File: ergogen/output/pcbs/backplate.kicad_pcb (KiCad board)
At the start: 2 copper layers, 139.5 x 113.2 mm, 5 parts

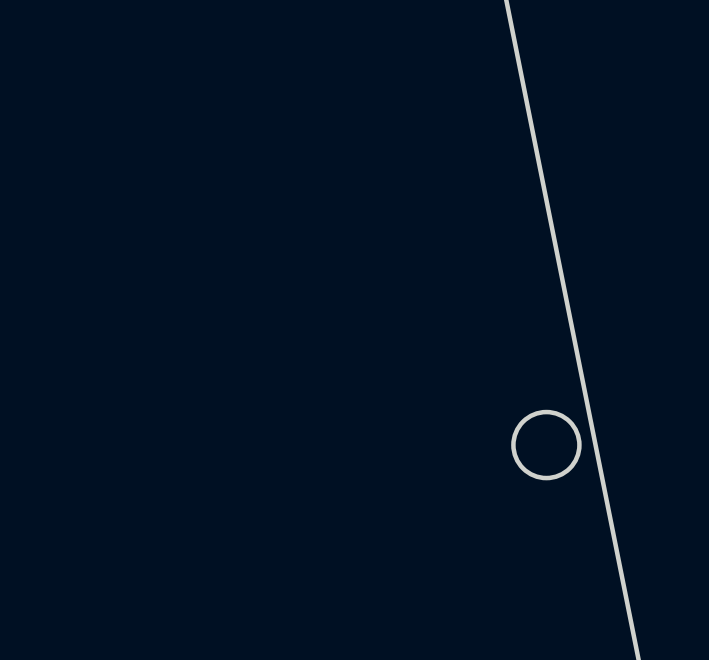
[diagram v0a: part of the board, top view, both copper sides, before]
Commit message: Checkpoint
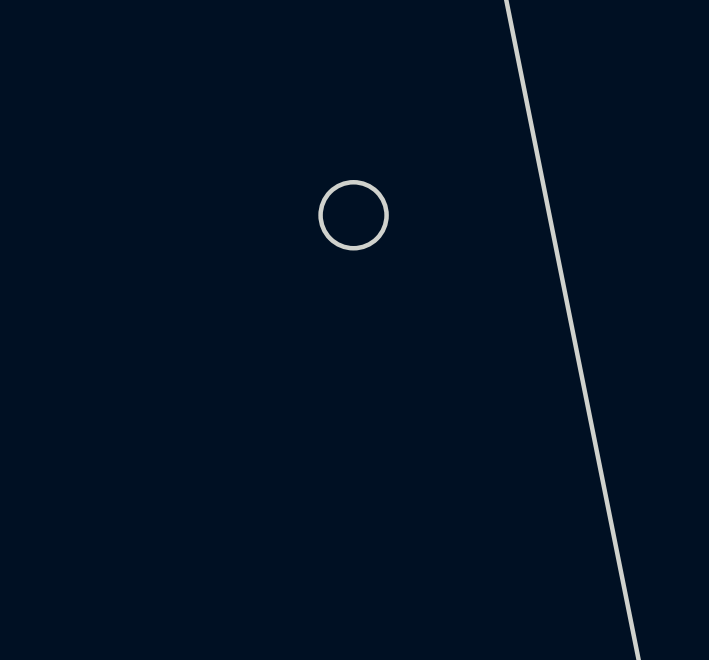
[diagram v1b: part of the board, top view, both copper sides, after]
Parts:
- moved MH5 10.00 mm to (220.8, 121.4)
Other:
- outline, holes or cut-outs redrawn
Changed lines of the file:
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@@
   )
   (module "ceoloide:mounting_hole_npth" (layer F.Cu)
-      (at 227.2307082 129.0614476 -50)
+      (at 220.8028321 121.40100319999999 -50)
       (fp_text reference "MH5" (at 0 2.55 -50) (layer F.SilkS) hide (effects (font (size 1 1) (thickness 0.15))))
       (pad "" np_thru_hole circle (at 0 0 -50) (size 2.2 2.2) (drill 2.2) (layers *.Cu *.Mask))
@@
 (gr_circle (center 185.468 61.361000000000004) (end 186.56799999999998 61.361000000000004) (layer Edge.Cuts) (width 0.15))
 (gr_circle (center 172.7442902 101.1746489) (end 173.8442902 101.1746489) (layer Edge.Cuts) (width 0.15))
-(gr_circle (center 227.2307082 129.0614476) (end 228.3307082 129.0614476) (layer Edge.Cuts) (width 0.15))
+(gr_circle (center 220.8028321 121.40100319999999) (end 221.90283209999998 121.40100319999999) (layer Edge.Cuts) (width 0.15))
 )

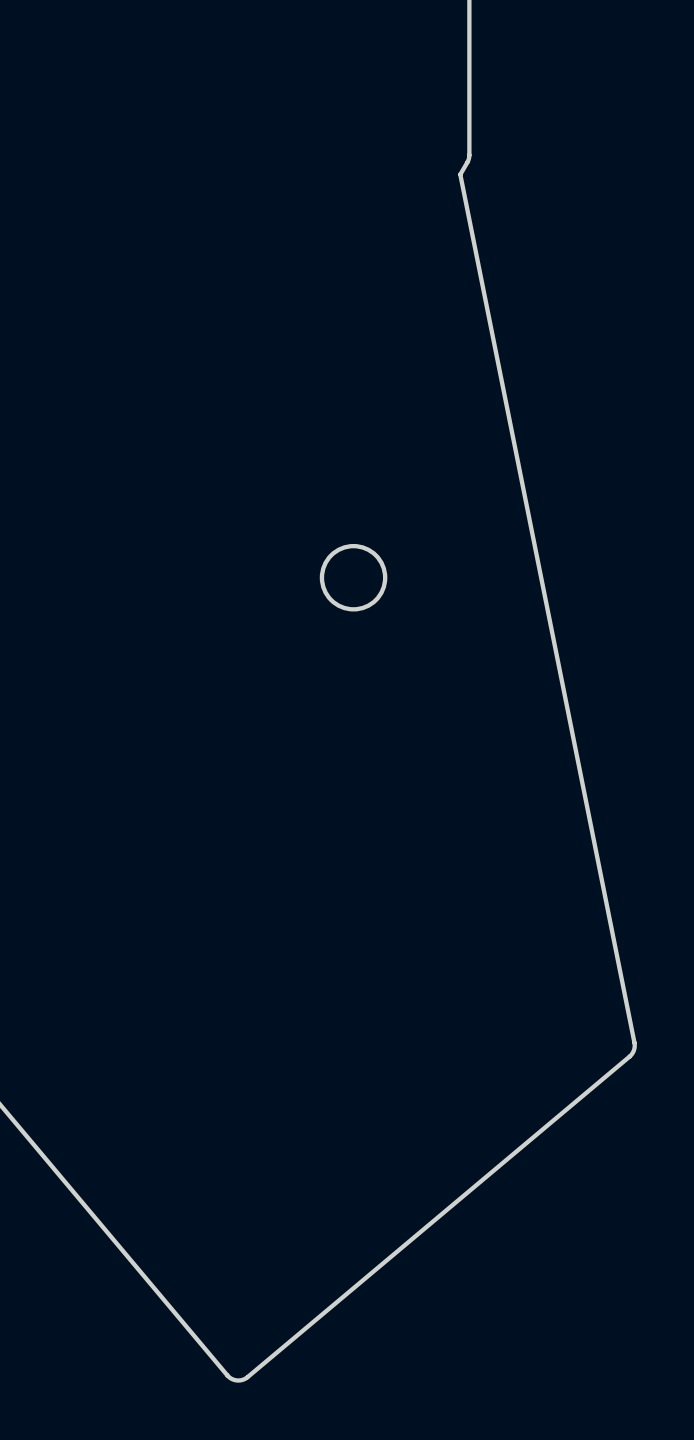
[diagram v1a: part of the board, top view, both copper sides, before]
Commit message: Checkpoint
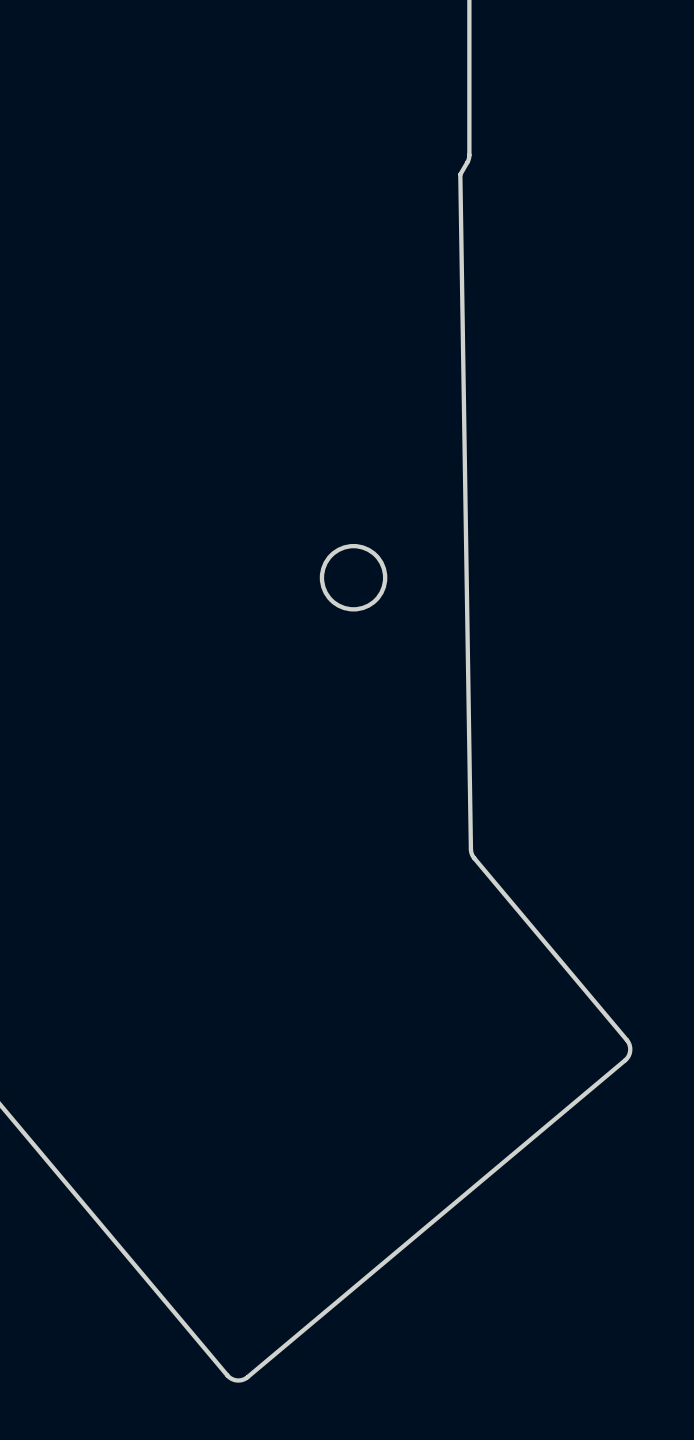
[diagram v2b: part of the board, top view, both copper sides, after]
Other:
- board size 139.5 x 113.2 mm -> 139.4 x 113.2 mm
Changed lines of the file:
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@@
 (gr_line (start 185.58186840000002 44.10813154431579) (end 203.5823534679014 44.1128685140705) (angle 90) (layer Edge.Cuts) (width 0.15))
 (gr_line (start 204.08222186790144 44.61264651408419) (end 204.08277807371226 45.86522200005129) (angle 90) (layer Edge.Cuts) (width 0.15))
-(gr_line (start 224.518 107.371596) (end 230.57788045934674 137.5834997388322) (angle 90) (layer Edge.Cuts) (width 0.15))
-(gr_line (start 230.40903856128045 138.06485304847308) (end 217.11551321531311 149.21944520216027) (angle 90) (layer Edge.Cuts) (width 0.15))
+(gr_line (start 224.518 107.371596) (end 224.88688692725793 130.84827901796234) (angle 90) (layer Edge.Cuts) (width 0.15))
+(gr_line (start 225.00380302725722 131.16181731796115) (end 230.3148039002676 137.491221684766) (angle 90) (layer Edge.Cuts) (width 0.15))
+(gr_line (start 230.25317550026756 138.19563768476607) (end 217.1155132153131 149.21944520216027) (angle 90) (layer Edge.Cuts) (width 0.15))
 (gr_line (start 216.41109721531305 149.1578168021602) (end 205.28039649130588 135.89276421578668) (angle 90) (layer Edge.Cuts) (width 0.15))
 (gr_line (start 205.18757259130587 135.8069910157867) (end 189.74612938848182 124.80148031587586) (angle 90) (layer Edge.Cuts) (width 0.15))
@@
 (gr_arc (start 224.333 46.865) (end 224.833 46.865) (angle -90) (layer Edge.Cuts) (width 0.15))
 (gr_arc (start 224.333 106.69202540612952) (end 224.7660127 106.94202540612952) (angle -30.000000108401252) (layer Edge.Cuts) (width 0.15))
-(gr_arc (start 230.0876447612805 137.68183084847306) (end 230.4090385612805 138.06485304847305) (angle -61.34183996214843) (layer Edge.Cuts) (width 0.15))
-(gr_arc (start 216.7941194153131 148.83642300216025) (end 216.4110972153131 149.15781680216026) (angle -90.00000000000713) (layer Edge.Cuts) (width 0.15))
+(gr_arc (start 225.3868252272579 130.84042351796052) (end 224.8868869272579 130.84827901796052) (angle -39.099790156987126) (layer Edge.Cuts) (width 0.15))
+(gr_arc (start 229.93178170026758 137.812615484766) (end 230.2531755002676 138.195637684766) (angle -90.00000000000456) (layer Edge.Cuts) (width 0.15))
+(gr_arc (start 216.79411941531308 148.83642300216025) (end 216.41109721531308 149.15781680216026) (angle -90.00000000000503) (layer Edge.Cuts) (width 0.15))
 (gr_arc (start 204.8973742913059 136.21415801578672) (end 205.2803964913059 135.8927642157867) (angle -14.521558200128908) (layer Edge.Cuts) (width 0.15))
 (gr_arc (start 189.45593108848183 125.20864731587585) (end 189.74612938848182 124.80148031587585) (angle -15.00000020686845) (layer Edge.Cuts) (width 0.15))

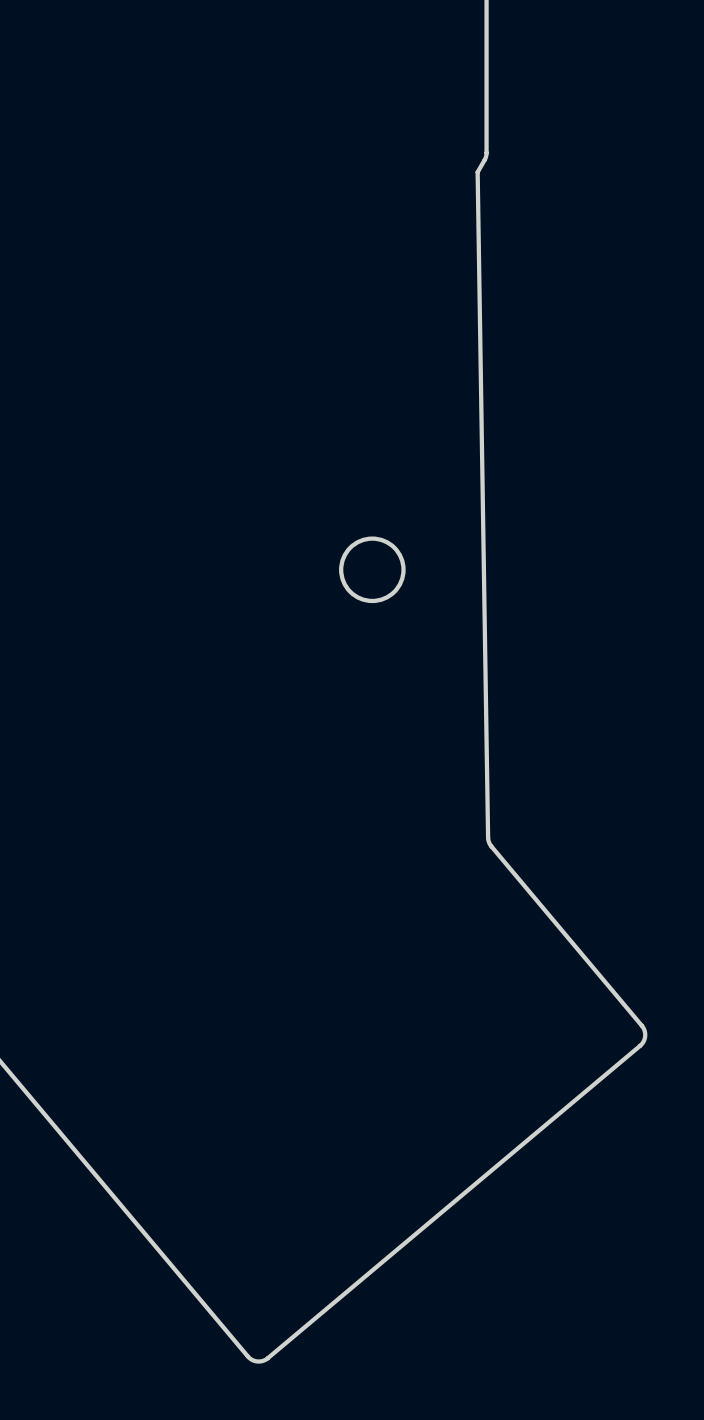
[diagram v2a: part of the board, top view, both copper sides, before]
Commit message: Checkpoint
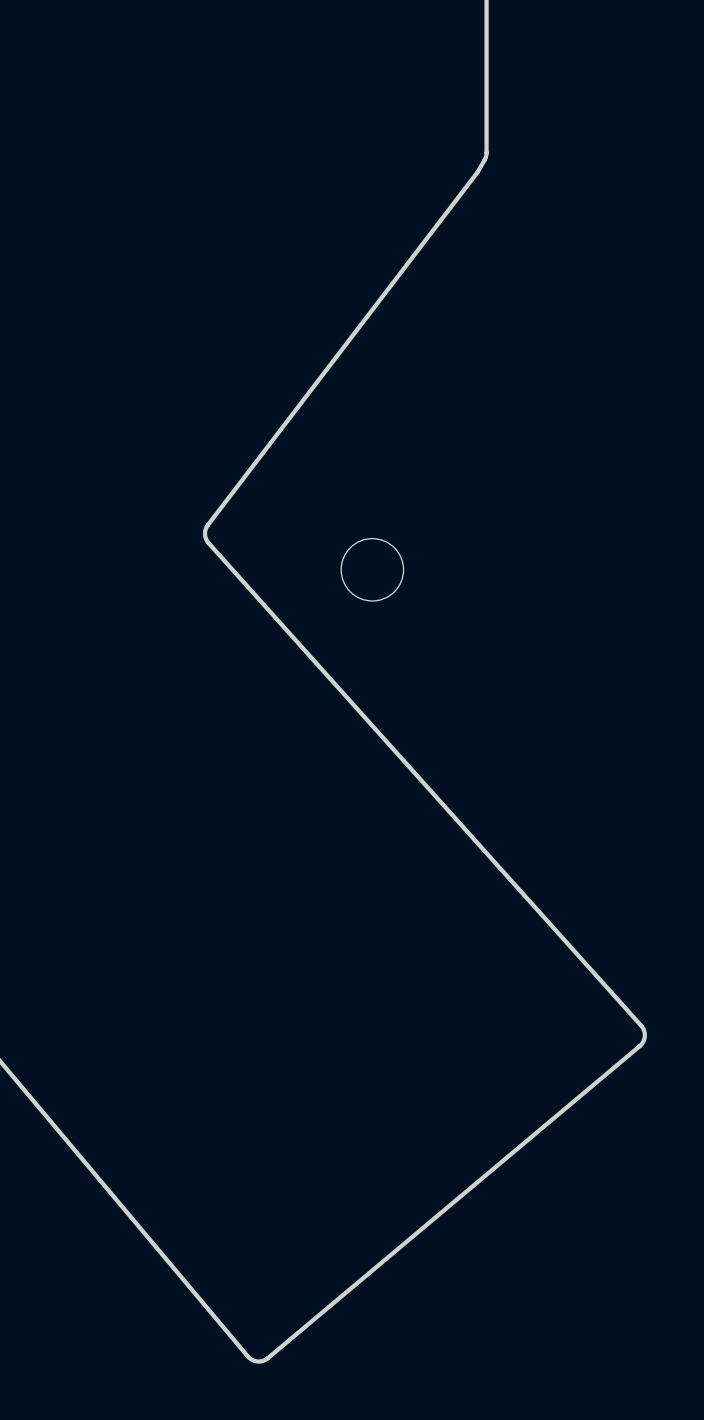
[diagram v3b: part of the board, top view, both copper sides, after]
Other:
- board size 139.4 x 113.2 mm -> 139.3 x 113.2 mm
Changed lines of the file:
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@@
 (gr_line (start 185.58186840000002 44.10813154431579) (end 203.5823534679014 44.1128685140705) (angle 90) (layer Edge.Cuts) (width 0.15))
 (gr_line (start 204.08222186790144 44.61264651408419) (end 204.08277807371226 45.86522200005129) (angle 90) (layer Edge.Cuts) (width 0.15))
-(gr_line (start 224.518 107.371596) (end 224.88688692725793 130.84827901796234) (angle 90) (layer Edge.Cuts) (width 0.15))
-(gr_line (start 225.00380302725722 131.16181731796115) (end 230.3148039002676 137.491221684766) (angle 90) (layer Edge.Cuts) (width 0.15))
-(gr_line (start 230.25317550026756 138.19563768476607) (end 217.1155132153131 149.21944520216027) (angle 90) (layer Edge.Cuts) (width 0.15))
+(gr_line (start 224.518 107.371596) (end 215.000872206663 119.8221967277347) (angle 90) (layer Edge.Cuts) (width 0.15))
+(gr_line (start 215.02579756409878 120.45958288341856) (end 230.29136629405417 137.4895566408562) (angle 90) (layer Edge.Cuts) (width 0.15))
+(gr_line (start 230.2404461940542 138.20631884085628) (end 217.11551321531311 149.21944520216024) (angle 90) (layer Edge.Cuts) (width 0.15))
 (gr_line (start 216.41109721531305 149.1578168021602) (end 205.28039649130588 135.89276421578668) (angle 90) (layer Edge.Cuts) (width 0.15))
 (gr_line (start 205.18757259130587 135.8069910157867) (end 189.74612938848182 124.80148031587586) (angle 90) (layer Edge.Cuts) (width 0.15))
@@
 (gr_arc (start 224.333 46.865) (end 224.833 46.865) (angle -90) (layer Edge.Cuts) (width 0.15))
 (gr_arc (start 224.333 106.69202540612952) (end 224.7660127 106.94202540612952) (angle -30.000000108401252) (layer Edge.Cuts) (width 0.15))
-(gr_arc (start 225.3868252272579 130.84042351796052) (end 224.8868869272579 130.84827901796052) (angle -39.099790156987126) (layer Edge.Cuts) (width 0.15))
-(gr_arc (start 229.93178170026758 137.812615484766) (end 230.2531755002676 138.195637684766) (angle -90.00000000000456) (layer Edge.Cuts) (width 0.15))
-(gr_arc (start 216.79411941531308 148.83642300216025) (end 216.41109721531308 149.15781680216026) (angle -90.00000000000503) (layer Edge.Cuts) (width 0.15))
+(gr_arc (start 215.39811146409875 120.12584288341856) (end 215.00087226409875 119.82219678341856) (angle -79.26683836697217) (layer Edge.Cuts) (width 0.15))
+(gr_arc (start 229.9190523940542 137.82329664085626) (end 230.24044619405421 138.20631884085626) (angle -91.8728626585997) (layer Edge.Cuts) (width 0.15))
+(gr_arc (start 216.7941194153131 148.83642300216025) (end 216.4110972153131 149.15781680216026) (angle -90.00000000000924) (layer Edge.Cuts) (width 0.15))
 (gr_arc (start 204.8973742913059 136.21415801578672) (end 205.2803964913059 135.8927642157867) (angle -14.521558200128908) (layer Edge.Cuts) (width 0.15))
 (gr_arc (start 189.45593108848183 125.20864731587585) (end 189.74612938848182 124.80148031587585) (angle -15.00000020686845) (layer Edge.Cuts) (width 0.15))
@@
 (gr_circle (center 185.468 61.361000000000004) (end 186.56799999999998 61.361000000000004) (layer Edge.Cuts) (width 0.15))
 (gr_circle (center 172.7442902 101.1746489) (end 173.8442902 101.1746489) (layer Edge.Cuts) (width 0.15))
-(gr_circle (center 220.8028321 121.40100319999999) (end 221.90283209999998 121.40100319999999) (layer Edge.Cuts) (width 0.15))
 )
